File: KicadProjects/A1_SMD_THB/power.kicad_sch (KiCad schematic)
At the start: 2 parts, among them P1 USB_C_Plug

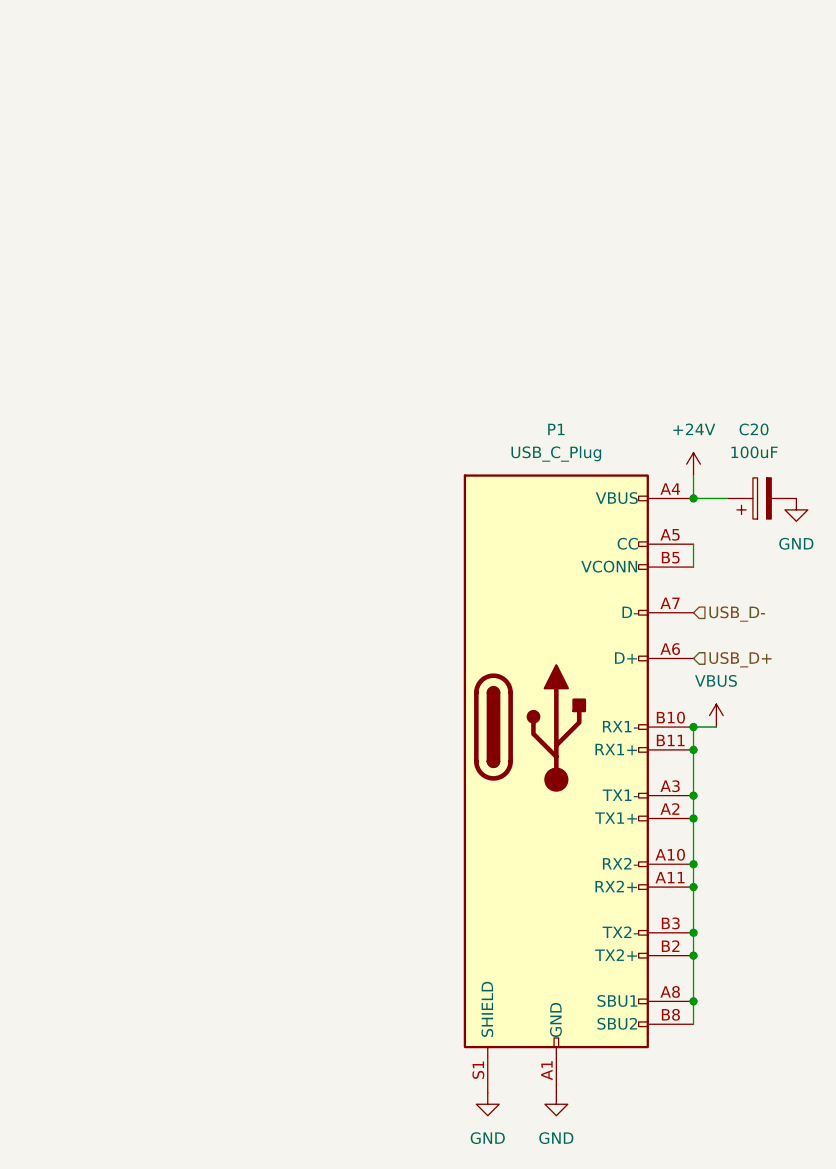
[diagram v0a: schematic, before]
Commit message: e
e
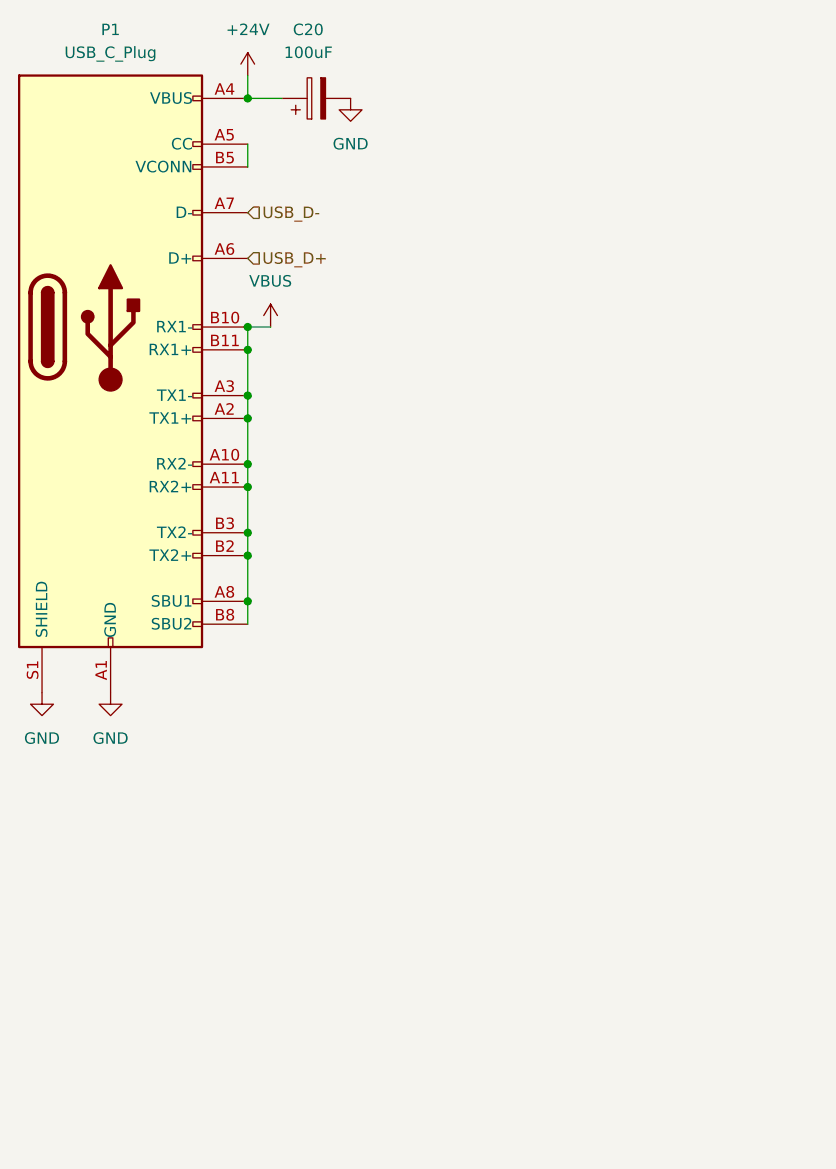
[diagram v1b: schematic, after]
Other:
- moved on the sheet: C20, P1

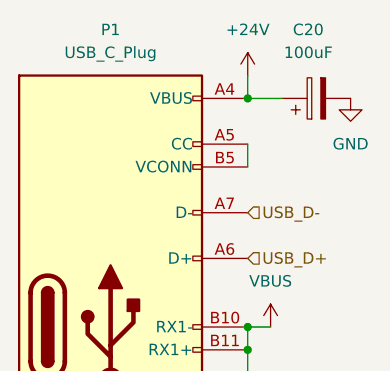
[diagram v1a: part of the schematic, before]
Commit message: e
e
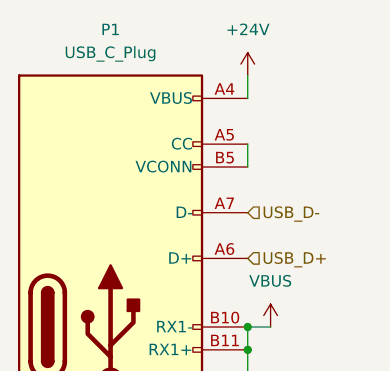
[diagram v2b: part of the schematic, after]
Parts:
- removed C20: 100uF, Capacitor_SMD:CP_Elec_8x10, symbol Device:C_Polarized
- P1: footprint Connector_USB:USB_C_Receptacle_G-Switch_GT-USB-7025 -> Connector_USB:USB_C_Receptacle_HCTL_HC-TYPE-C-16P-01A
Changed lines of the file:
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@@
-	)
-	(junction
-		(at 64.77 39.37)
-		(diameter 0)
-		(color 0 0 0 0)
 	)
 	(junction
@@
 		(pts
 			(xy 64.77 82.55) (xy 64.77 87.63)
-		)
-		(stroke
-			(width 0)
-			(type default)
-		)
-	)
-	(wire
-		(pts
-			(xy 64.77 39.37) (xy 68.58 39.37)
 		)
 		(stroke
@@
 	)
 	(symbol
-		(lib_id "Device:C_Polarized")
-		(at 72.39 39.37 90)
-		(unit 1)
-		(exclude_from_sim no)
-		(in_bom yes)
-		(on_board yes)
-		(dnp no)
-		(fields_autoplaced yes)
-		(property "Reference" "C20"
-			(at 71.501 31.75 90)
-			(effects
-				(font
-					(size 1.27 1.27)
-				)
-			)
-		)
-		(property "Value" "100uF"
-			(at 71.501 34.29 90)
-			(effects
-				(font
-					(size 1.27 1.27)
-				)
-			)
-		)
-		(property "Footprint" "Capacitor_SMD:CP_Elec_8x10"
-			(at 76.2 38.4048 0)
-			(effects
-				(font
-					(size 1.27 1.27)
-				)
-				(hide yes)
-			)
-		)
-		(property "Datasheet" "~"
-			(at 72.39 39.37 0)
-			(effects
-				(font
-					(size 1.27 1.27)
-				)
-				(hide yes)
-			)
-		)
-		(property "Description" "Polarized capacitor"
-			(at 72.39 39.37 0)
-			(effects
-				(font
-					(size 1.27 1.27)
-				)
-				(hide yes)
-			)
-		)
-		(pin "1"
-		)
-		(pin "2"
-		)
-		(instances
-			(project "A1_SMD_THB"
-				(path "/34183abe-6288-4424-a0b3-d63b1476ac75/85a00ac2-5790-47c0-90dd-4eac1528d388"
-					(reference "C20")
-					(unit 1)
-				)
-			)
-		)
-	)
-	(symbol
 		(lib_id "power:+24V")
 		(at 64.77 36.83 0)
@@
 			)
 		)
-		(property "Footprint" "Connector_USB:USB_C_Receptacle_G-Switch_GT-USB-7025"
+		(property "Footprint" "Connector_USB:USB_C_Receptacle_HCTL_HC-TYPE-C-16P-01A"
 			(at 53.34 64.77 0)
 			(effects
@@
 					(unit 1)
 				)
-			)
-		)
-	)
-	(symbol
-		(lib_id "power:GND")
-		(at 76.2 39.37 0)
-		(unit 1)
-		(exclude_from_sim no)
-		(in_bom yes)
-		(on_board yes)
-		(dnp no)
-		(fields_autoplaced yes)
-		(property "Reference" "#PWR030"
-			(at 76.2 45.72 0)
-			(effects
-				(font
-					(size 1.27 1.27)
-				)
-				(hide yes)
-			)
-		)
-		(property "Value" "GND"
-			(at 76.2 44.45 0)
-			(effects
-				(font
-					(size 1.27 1.27)
-				)
-			)
-		)
-		(property "Footprint" ""
-			(at 76.2 39.37 0)
-			(effects
-				(font
-					(size 1.27 1.27)
-				)
-				(hide yes)
-			)
-		)
-		(property "Datasheet" ""
-			(at 76.2 39.37 0)
-			(effects
-				(font
-					(size 1.27 1.27)
-				)
-				(hide yes)
-			)
-		)
-		(property "Description" "Power symbol creates a global label with name \"GND\" , ground"
-			(at 76.2 39.37 0)
-			(effects
-				(font
-					(size 1.27 1.27)
-				)
-				(hide yes)
-			)
-		)
-		(pin "1"
-		)
-		(instances
-			(project "A1_SMD_THB"
-				(path "/34183abe-6288-4424-a0b3-d63b1476ac75/85a00ac2-5790-47c0-90dd-4eac1528d388"
-					(reference "#PWR030")
-					(unit 1)
-				)
